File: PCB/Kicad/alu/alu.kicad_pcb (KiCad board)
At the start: 2 copper layers, 200 x 100 mm, 230 parts, among them J1 out, J2 out, U1 7408, U10 7408, U11 7486, U12 7486, U13 7486, U14 7486, U15 7404, U16 7404, U17 7486, U18 7486, U19 7486, U2 7404, U20 74283, U21 74283, U22 7486, U23 7486, U24 74283, U25 74283, U26 74257, U27 74257, U28 74257, U29 74257, U3 7432, U30 74257, U31 74257, U32 74257, U33 74257, U34 74257, U35 74257, U36 74257, U37 74257, U38 74257, U39 74257, U4 7432, U40 74257, U41 74257, U42 74257, U43 74257, U44 74257, U45 74257, U46 74257, U47 74257, U48 74257, U49 74257, U5 7432, U50 74377, U51 74377, U52 74245, U53 74245, U54 74139, U55 7432, U56 7432, U57 7432, U58 74377, U59 74377, U6 7432, U60 74245, U61 74245, U62 74245, U63 74245, U64 74245, U65 74245, U66 74245, U67 74245, U68 74245, U69 74245, U7 7408, U70 7432, U71 7486, U72 7432, U73 7404, U74 7432, U75 7408, U8 7408, U9 7408

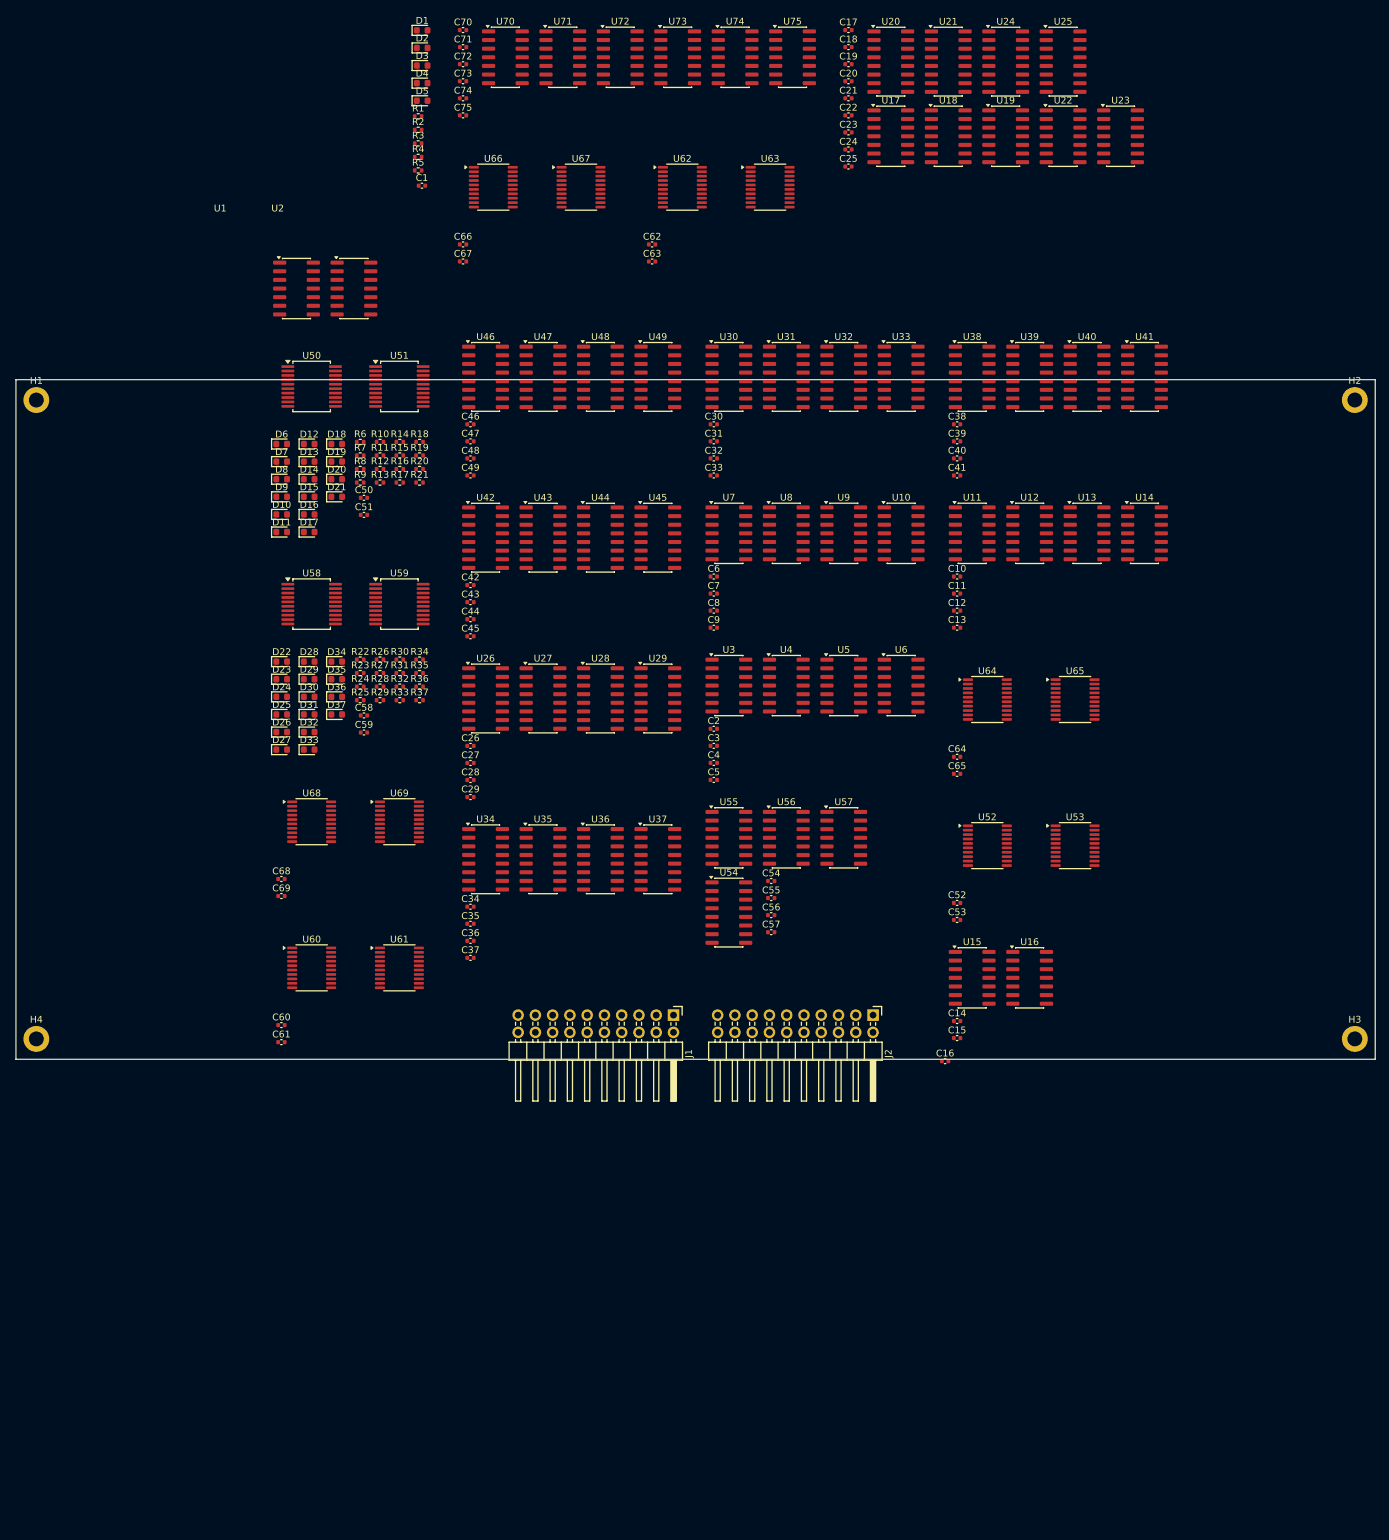
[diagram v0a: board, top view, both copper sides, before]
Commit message: alu board adjustement
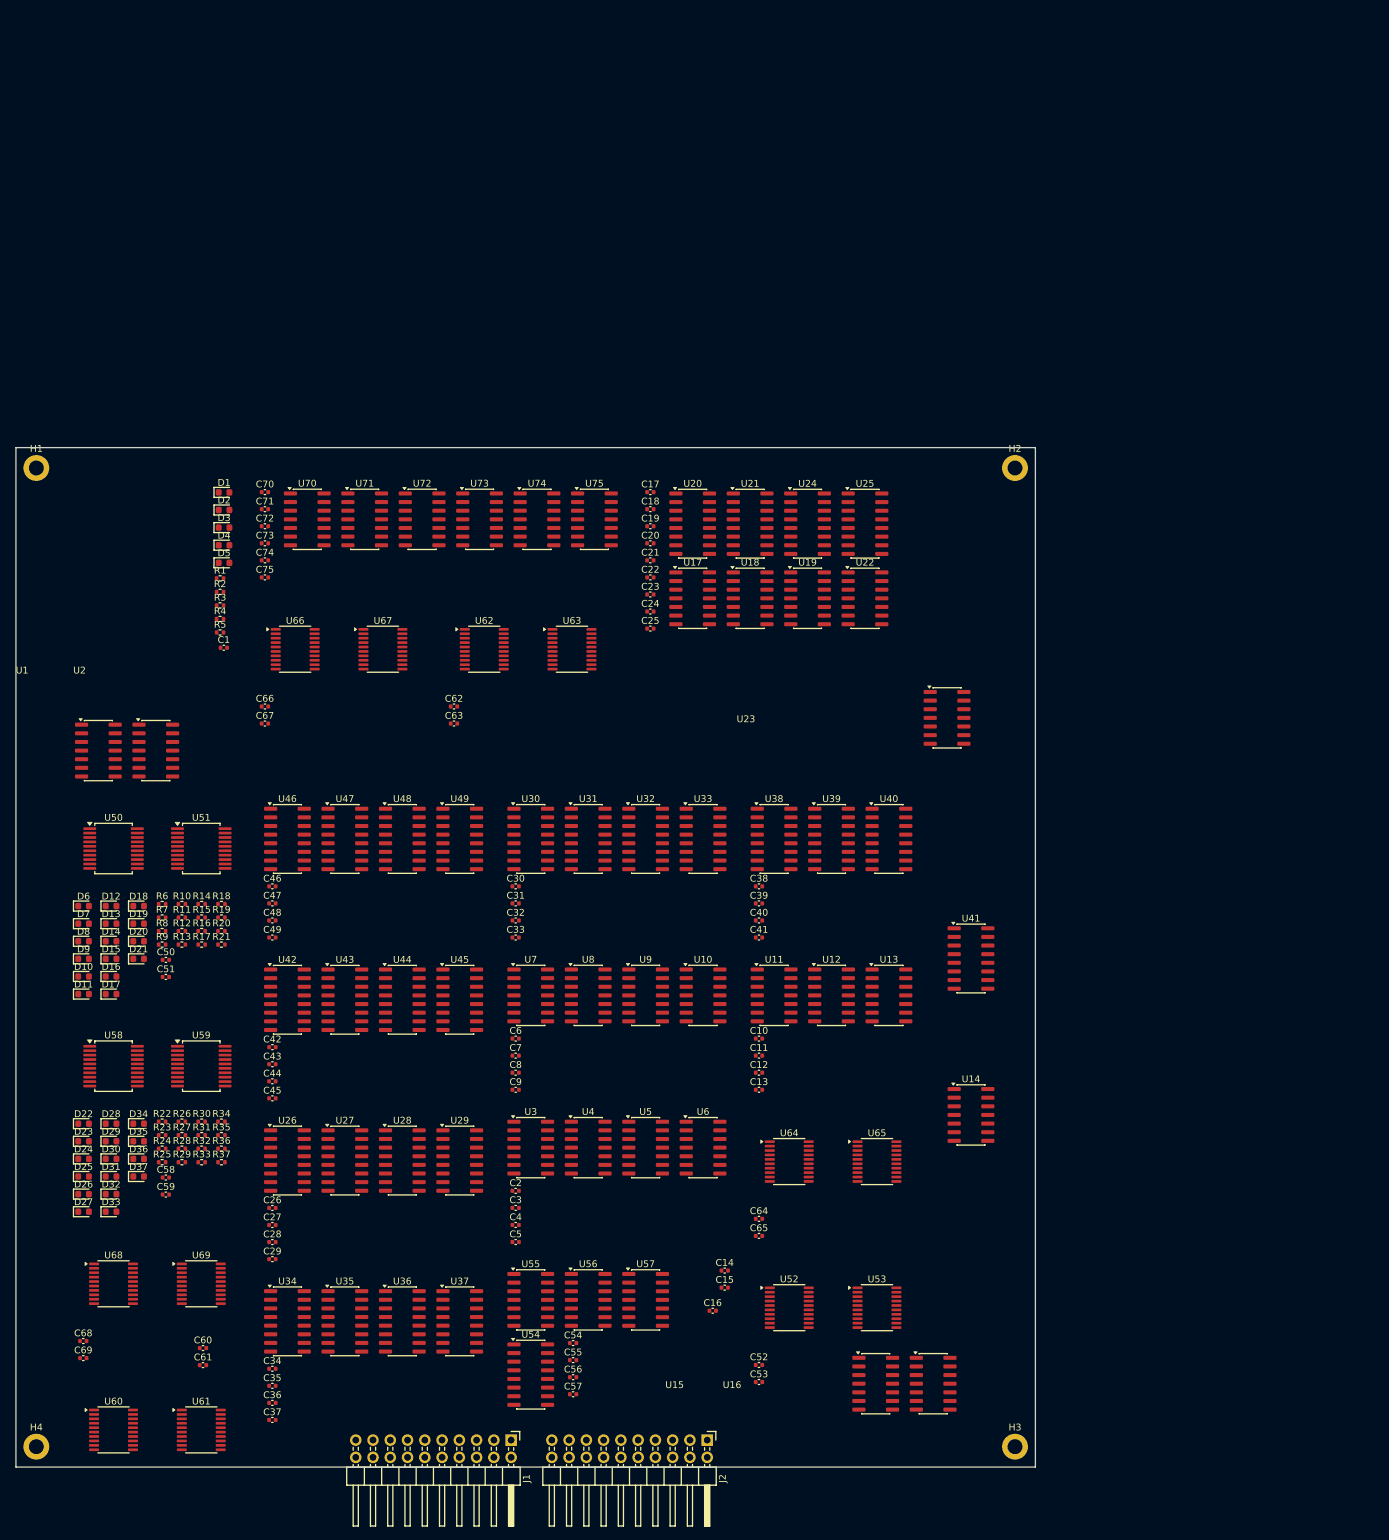
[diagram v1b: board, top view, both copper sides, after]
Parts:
- moved U23 89.3 mm to (157.0, 69.8)
- moved U41 89.3 mm to (160.5, 105.2)
- moved U14 89.3 mm to (160.5, 128.2)
- moved H3 78.1 mm to (167.0, 177.0)
- moved C3 74.0 mm to (93.5, 141.9)
- moved C30 74.0 mm to (93.5, 94.6)
- moved C7 74.0 mm to (93.5, 119.5)
- moved D20 74.0 mm to (38.0, 102.6)
- moved R16 74.0 mm to (47.3, 101.1)
- moved R30 74.0 mm to (47.3, 129.2)
- moved R33 74.0 mm to (47.3, 135.1)
- moved U52 74.0 mm to (133.8, 156.6)
- moved U53 74.0 mm to (146.7, 156.6)
- moved U64 74.0 mm to (133.8, 135.1)
- moved U65 74.0 mm to (146.7, 135.1)
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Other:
- board size 200 x 100 mm -> 150 x 150 mm
